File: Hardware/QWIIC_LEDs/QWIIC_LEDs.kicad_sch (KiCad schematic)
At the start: 25 parts, among them J1 SWD CONNECTOR, J2 QWIIC, U1 ATtiny1616-M

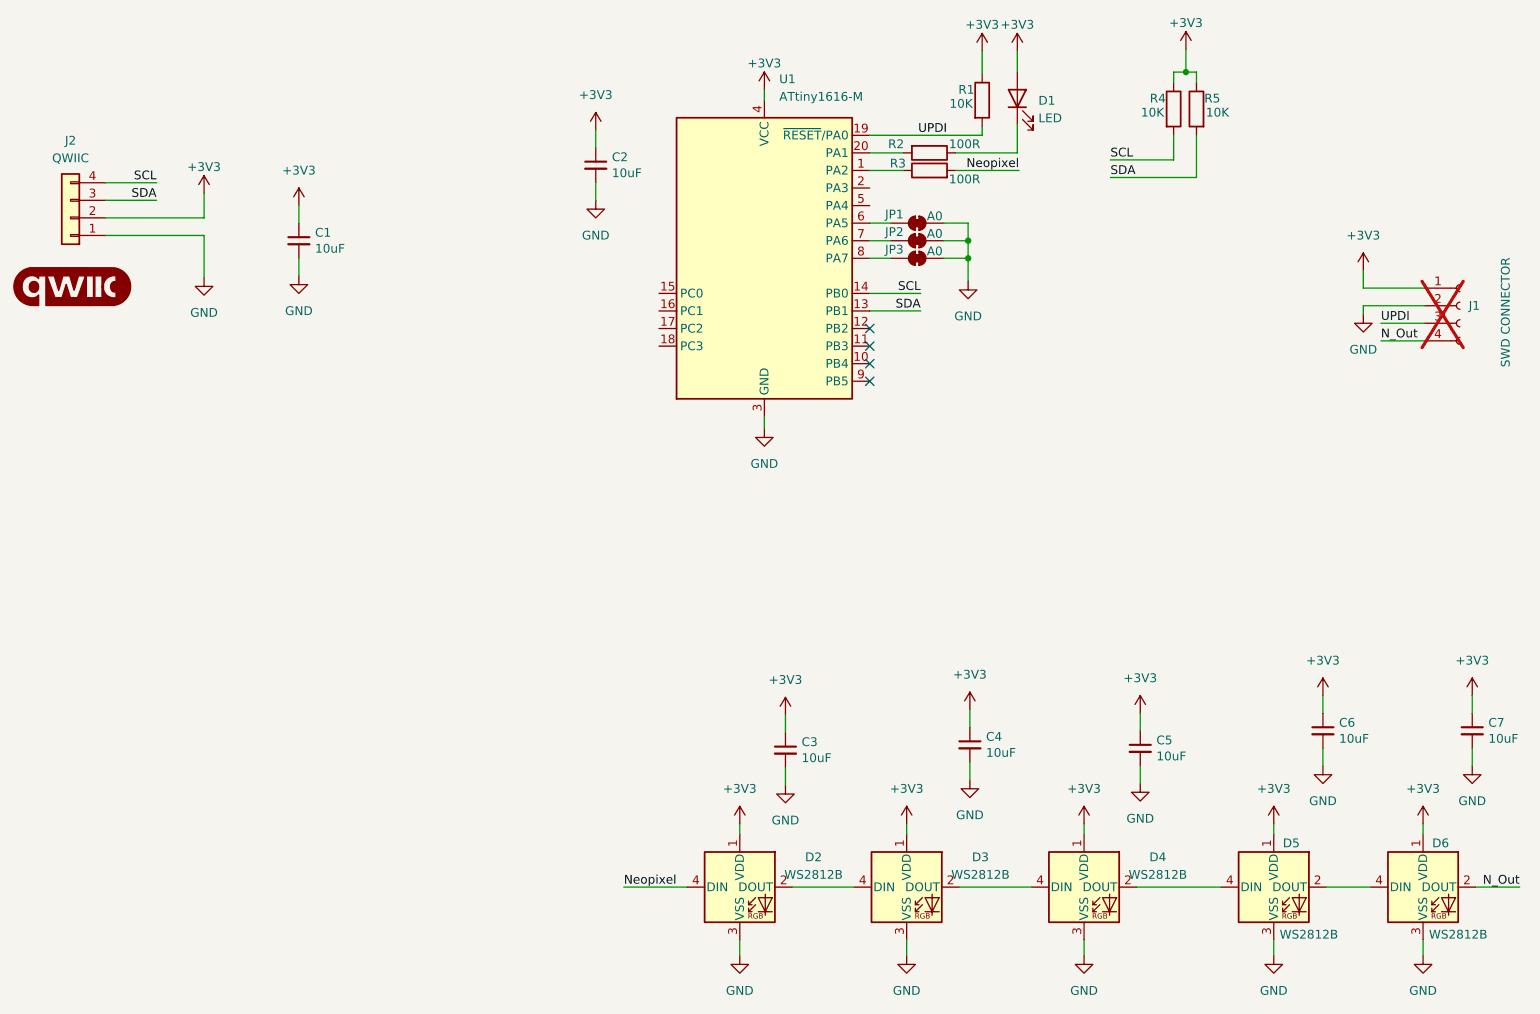
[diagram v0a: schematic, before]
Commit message: Update boms
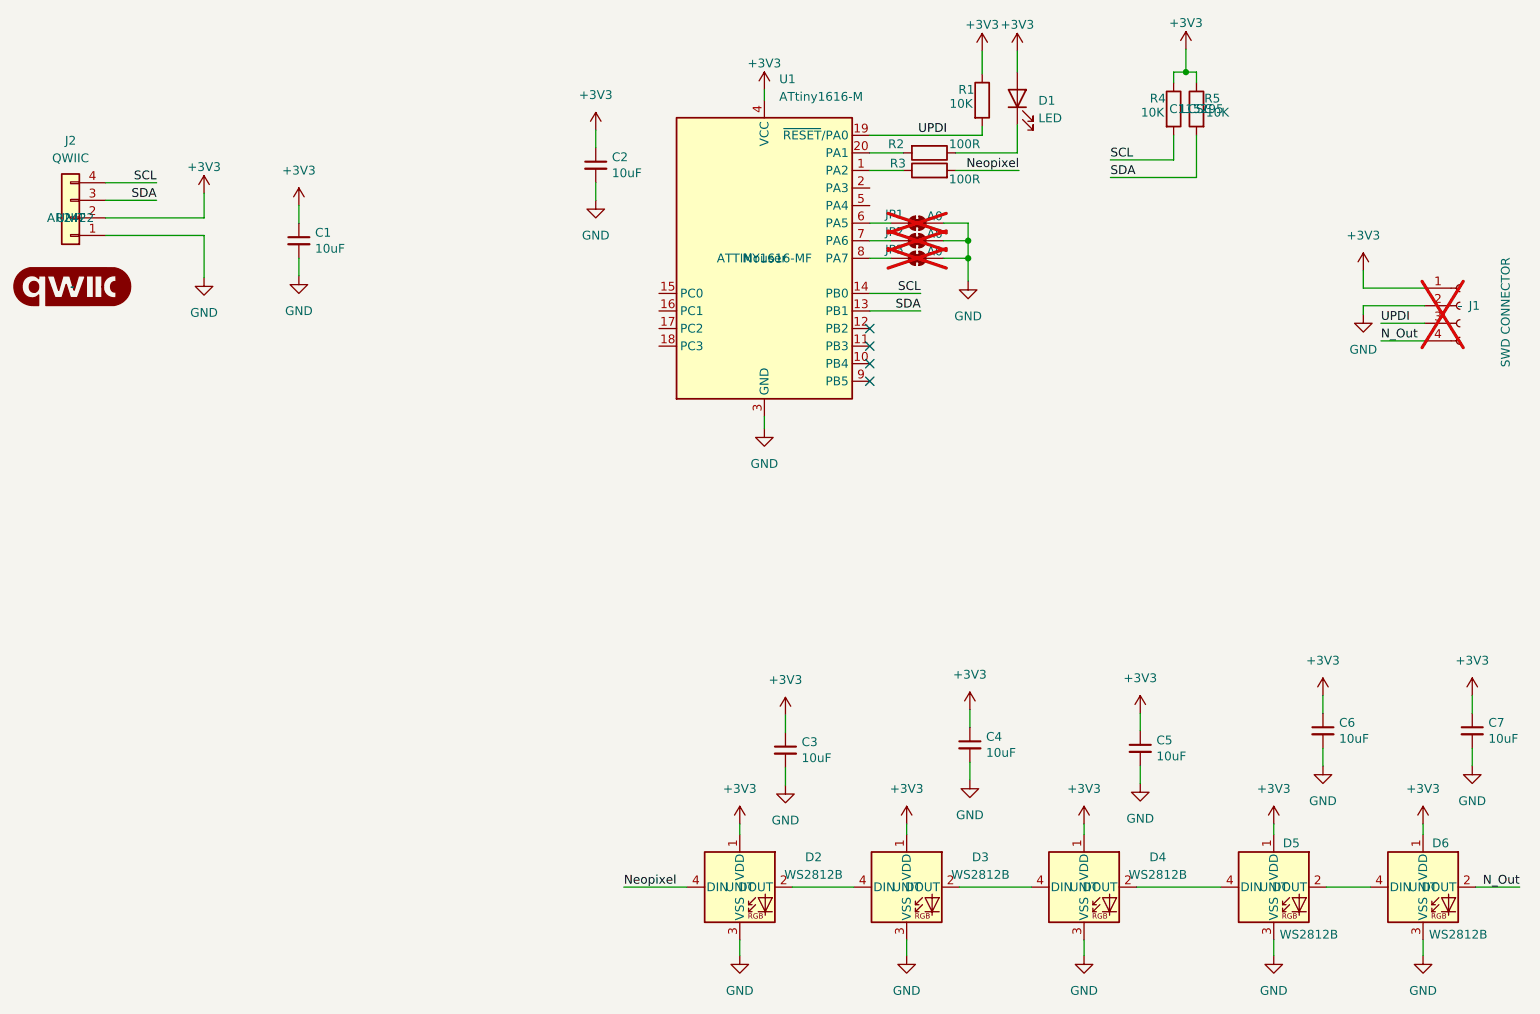
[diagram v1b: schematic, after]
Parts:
- C1, C2, C3, C4, C5, C6, C7: LCSC# C85713 -> C1713
- D1: manf# (none) -> 150080BS75000; provedor (none) -> Mouser
- D2, D3, D4, D5, D6: manf# WS2812B-B/W -> AR2232; provedor (none) -> UNIT
- G1, J1: manf# (none) -> -; provedor (none) -> -
- J2: manf# (none) -> AR2422; provedor (none) -> UNIT
- JP1, JP2, JP3: provedor (none) -> -; now not fitted
- R1, R4, R5: LCSC# (none) -> C115295; provedor (none) -> LCSC
- R2, R3: LCSC# (none) -> C106949; provedor (none) -> LCSC
- U1: manf# (none) -> ATTINY1616-MF; provedor (none) -> Mouser
